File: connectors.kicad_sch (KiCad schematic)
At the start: 27 parts, among them J12 Conn_01x02, J13 Conn_01x02, J15 Conn_01x08, J16 Conn_01x08, J17 Conn_01x08, J18 VIN, J19 USB_C_Receptacle_PowerOnly_6P, J5 Conn_01x02, J6 Conn_01x02, J7 Conn_01x02, J8 Conn_01x02, P1 USB_C_Plug_USB2.0, P2 USB_C_Plug_USB2.0

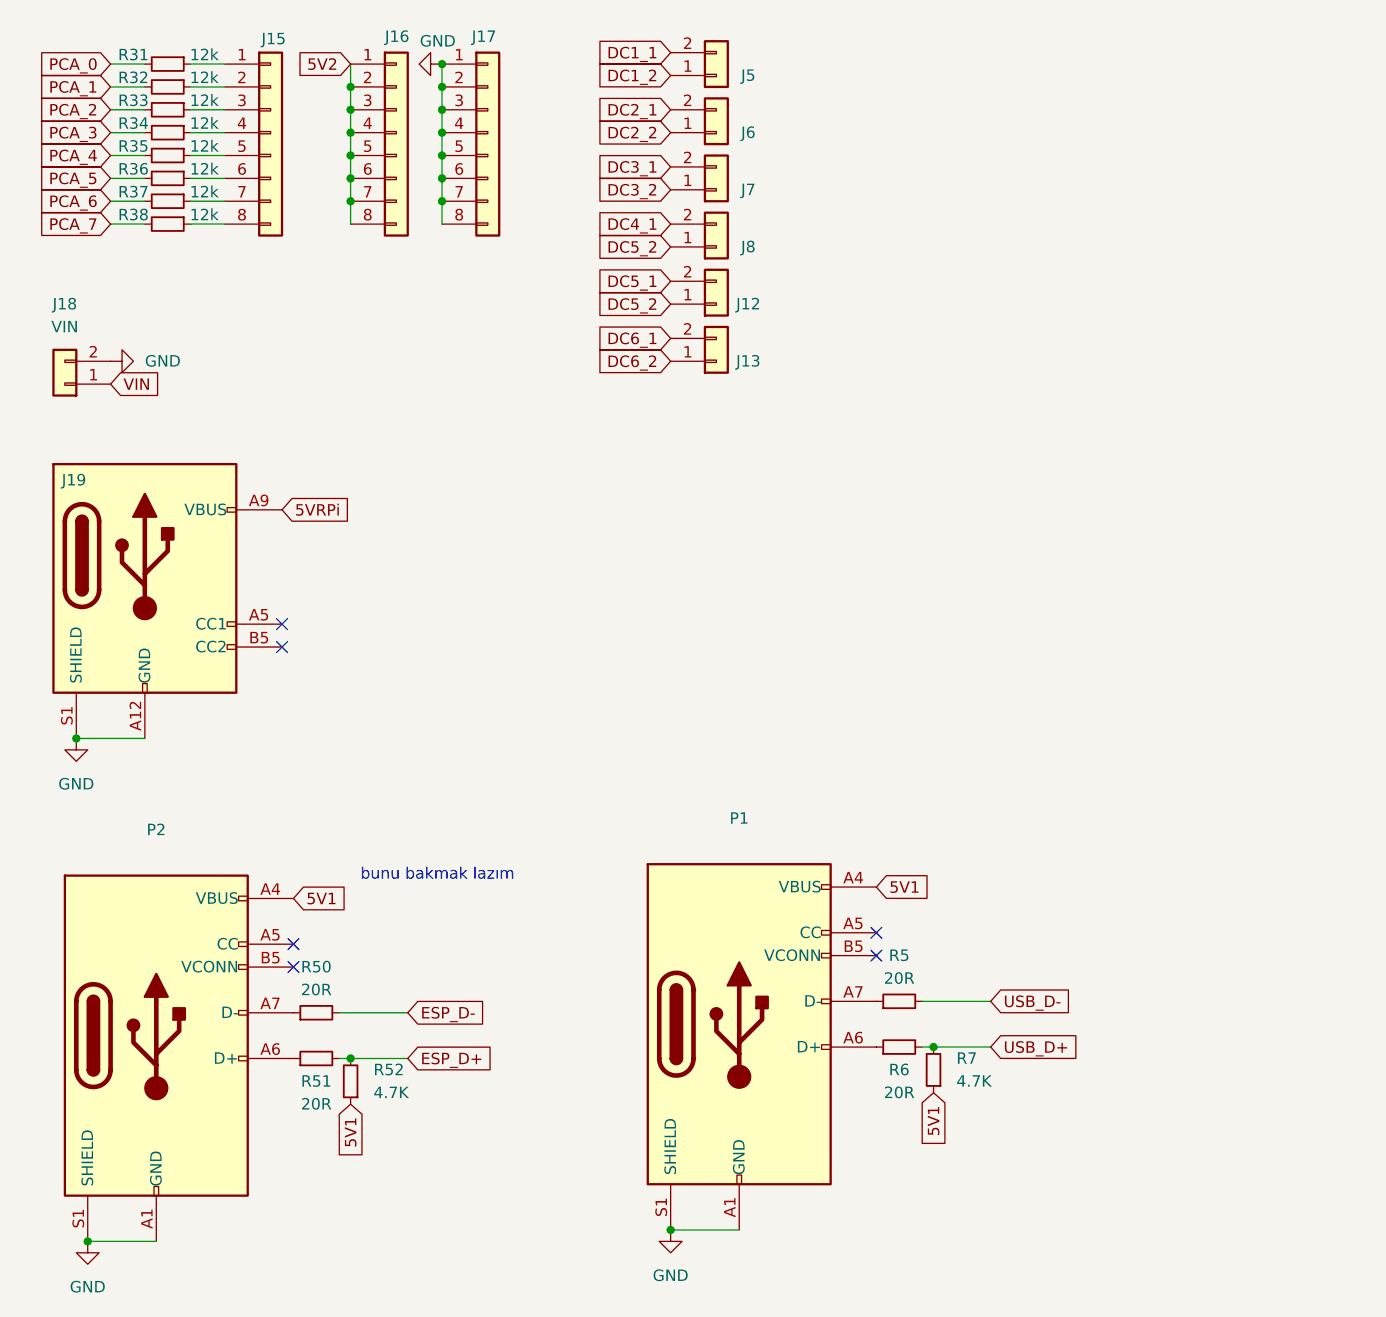
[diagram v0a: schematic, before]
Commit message: Visual Improvements
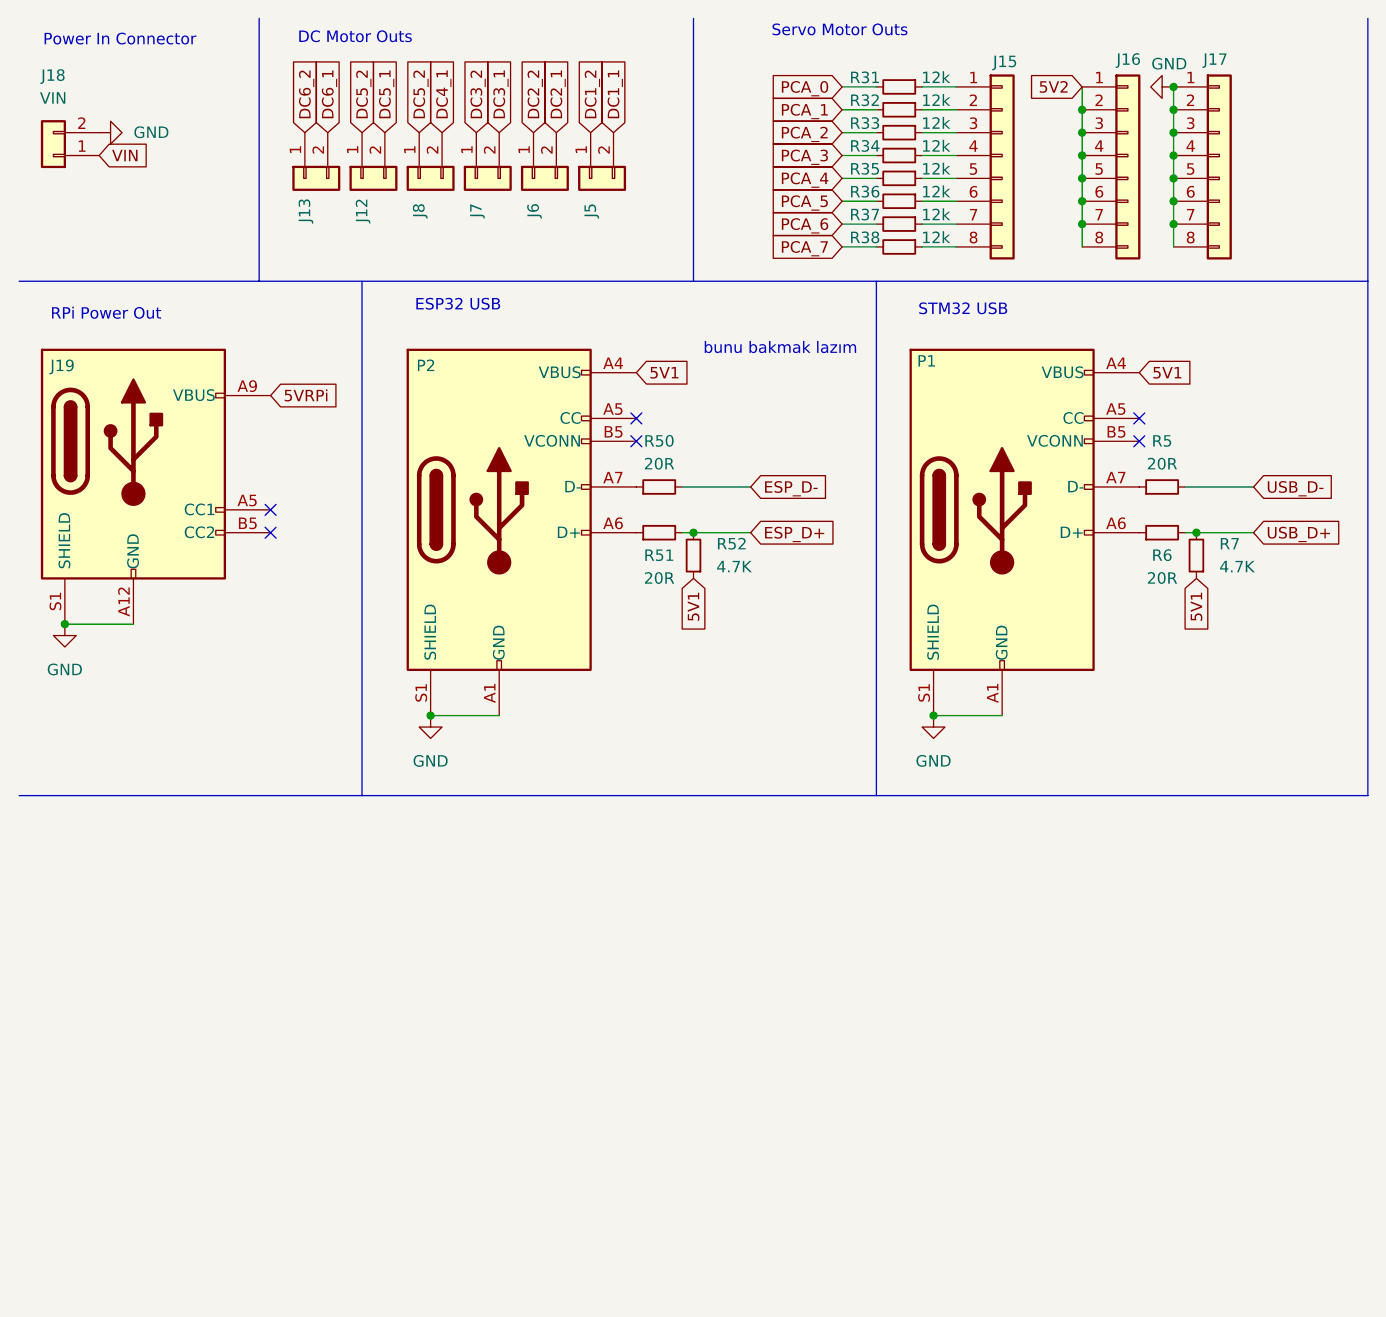
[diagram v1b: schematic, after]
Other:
- note added: "DC Motor Outs"
- note added: "ESP32 USB"
- note added: "Power In Connector"
- note added: "RPi Power Out"
- note added: "STM32 USB"
- note added: "Servo Motor Outs"
- moved on the sheet: J12, J13, J15, J16, J17, J18, J19, J5, J6, J7, J8, P1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
